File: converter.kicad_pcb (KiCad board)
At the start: 2 copper layers, 26.4 x 49.9 mm, 69 parts, among them CN1 MINI_DIN_8P_JACK, J1 USB_B, J2 USB_microB, SW1 SW_PUSH, U1 ATMEGA32U4, X1 16MHz

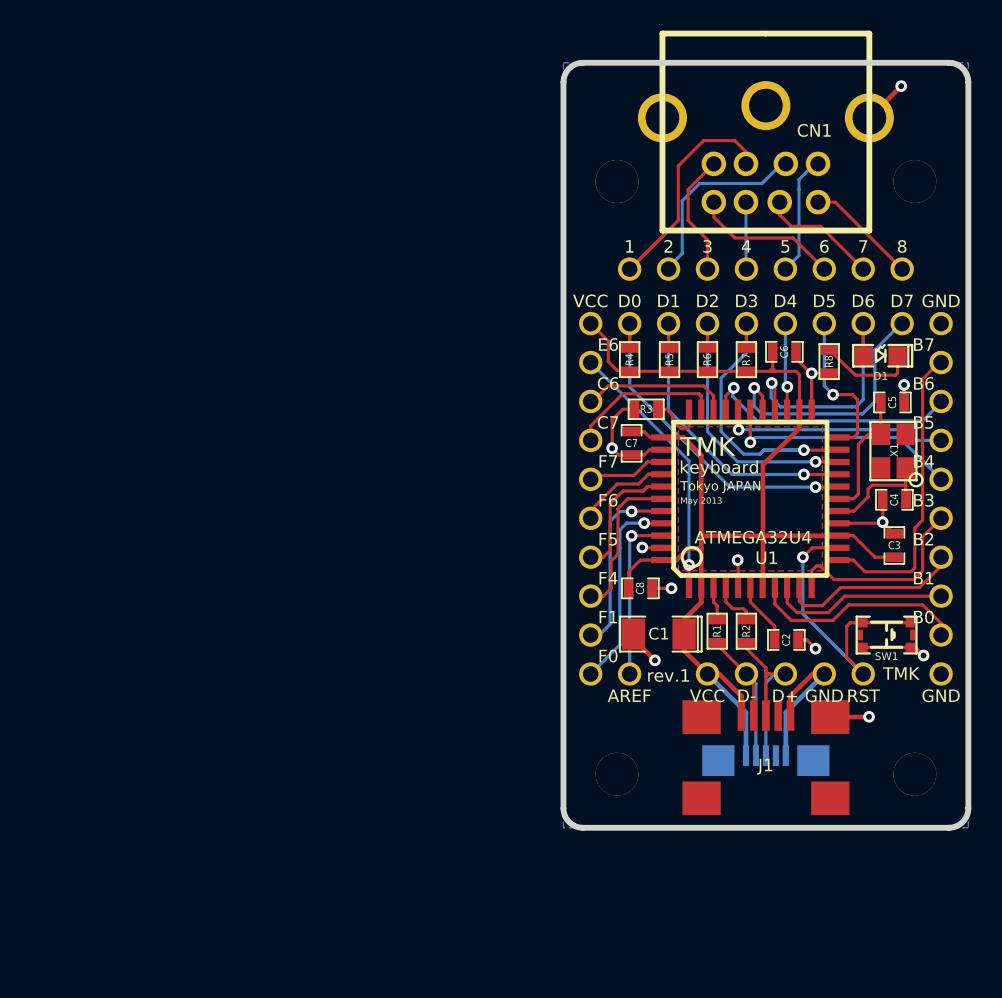
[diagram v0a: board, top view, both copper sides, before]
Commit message: Initial commit of PCB rev.2
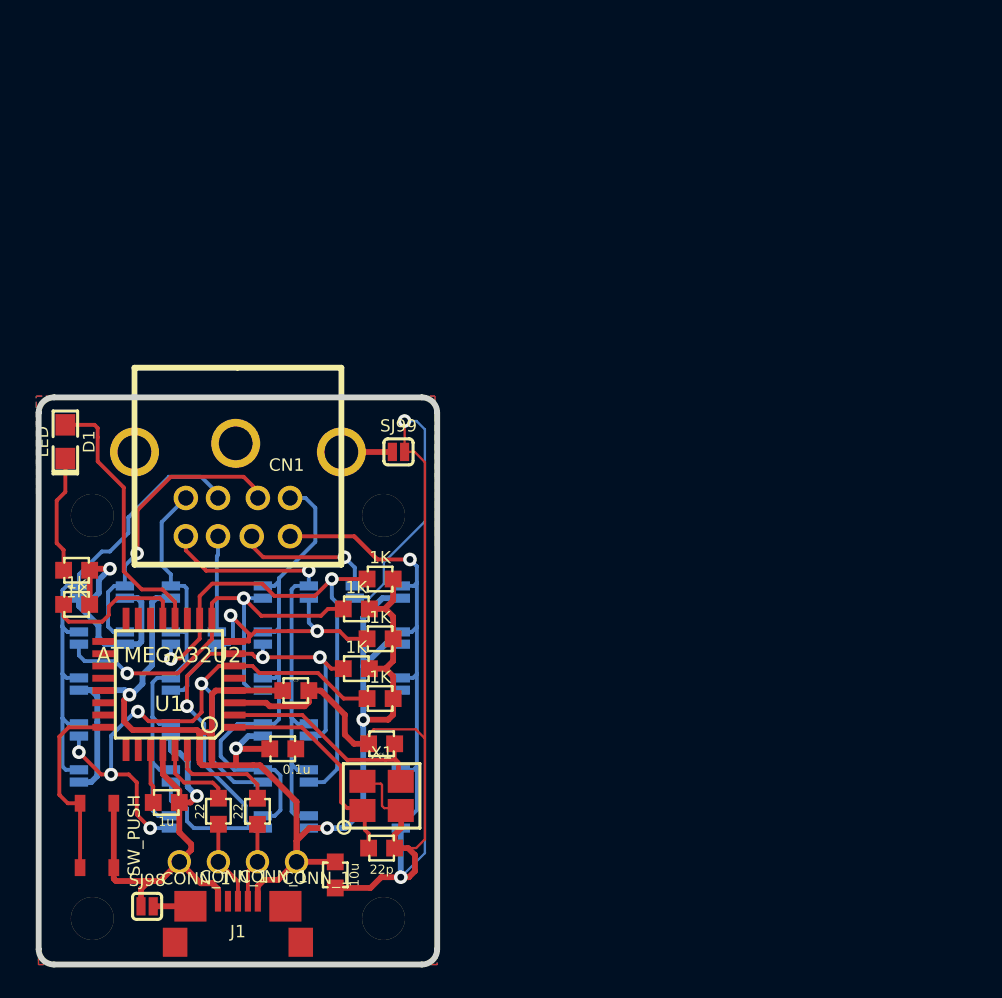
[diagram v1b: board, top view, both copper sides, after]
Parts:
- removed 1, 2, 3, 4, 5, 6, 7, 8, AREF, B0, B1, B2, B3, B4, B5, B6, B7, C7, D+, D-, D0, D2, D3, D4, D5, D6, D7, E6, F0, F1, F4, F5, F6, F7, GND (x3), RST, VCC (x2): CONN_1, PIN_1
- removed the C6 at (136.0, 100.3)
- removed the C6 at (148.7, 97.0)
- removed C7, C8: 0.1u, SM0603_Capa
- removed the D1 at (154.9, 97.3)
- removed the D1 at (141.1, 95.2)
- removed the HOLE_M2.6 at (157.2, 124.6)
- removed the HOLE_M2.6 at (137.7, 85.9)
- removed the HOLE_M2.6 at (157.2, 85.9)
- removed the HOLE_M2.6 at (137.7, 124.6)
- removed J2: USB_microB, USB_microB
- removed R5, R6, R7, R8: 1K, SM0603
- added C6: 22p, 000NewKeyboard_parts:C_1608, F.Cu at (122.4, 122.6)
- added D1: LED, 000NewKeyboard_parts:LED_0805, F.Cu at (101.7, 102.9)
- added HOLE_M2.6: VAL**, HOLE_M2.6, F.Cu at (123.0, 134.0)
- added HOLE_M2.6: VAL**, HOLE_M2.6, F.Cu at (103.4, 107.7)
- added HOLE_M2.6: VAL**, HOLE_M2.6, F.Cu at (122.9, 107.7)
- added HOLE_M2.6: VAL**, HOLE_M2.6, F.Cu at (103.5, 134.0)
- added P1: CONN_1, 000NewKeyboard_parts:PIN_1, F.Cu at (116.8, 130.3)
- added P2: CONN_1, 000NewKeyboard_parts:PIN_1, F.Cu at (114.3, 130.3)
- added P3: CONN_1, 000NewKeyboard_parts:PIN_1, F.Cu at (111.7, 130.3)
- added P4: CONN_1, 000NewKeyboard_parts:PIN_1, F.Cu at (109.2, 130.3)
- added R10: 1K, 000NewKeyboard_parts:R_1608, F.Cu at (122.3, 119.7)
- added R11: 1K, 000NewKeyboard_parts:R_1608, F.Cu at (120.7, 117.7)
- added R12: 1K, 000NewKeyboard_parts:R_1608, F.Cu at (122.3, 115.8)
- added R13: 1K, 000NewKeyboard_parts:R_1608, F.Cu at (120.7, 113.8)
- added R14: 1K, 000NewKeyboard_parts:R_1608, F.Cu at (122.3, 111.8)
- added SJ1: SOLDER_JUMPER, 000NewKeyboard_parts:SOLDER_JUMPER_2, B.Cu at (102.6, 112.7)
- added SJ10: SOLDER_JUMPER, 000NewKeyboard_parts:SOLDER_JUMPER_2, B.Cu at (108.6, 118.7)
- added SJ11: SOLDER_JUMPER, 000NewKeyboard_parts:SOLDER_JUMPER_2, B.Cu at (108.6, 121.7)
- added SJ12: SOLDER_JUMPER, 000NewKeyboard_parts:SOLDER_JUMPER_2, B.Cu at (108.6, 124.7)
- added SJ13: SOLDER_JUMPER, 000NewKeyboard_parts:SOLDER_JUMPER_2, B.Cu at (108.6, 127.7)
- added SJ14: SOLDER_JUMPER, 000NewKeyboard_parts:SOLDER_JUMPER_2, B.Cu at (111.6, 115.7)
- added SJ15: SOLDER_JUMPER, 000NewKeyboard_parts:SOLDER_JUMPER_2, B.Cu at (114.6, 112.7)
- added SJ16: SOLDER_JUMPER, 000NewKeyboard_parts:SOLDER_JUMPER_2, B.Cu at (114.6, 115.7)
- added SJ17: SOLDER_JUMPER, 000NewKeyboard_parts:SOLDER_JUMPER_2, B.Cu at (114.6, 118.7)
- added SJ18: SOLDER_JUMPER, 000NewKeyboard_parts:SOLDER_JUMPER_2, B.Cu at (114.6, 121.7)
- added SJ19: SOLDER_JUMPER, 000NewKeyboard_parts:SOLDER_JUMPER_2, B.Cu at (114.6, 124.7)
- added SJ2: SOLDER_JUMPER, 000NewKeyboard_parts:SOLDER_JUMPER_2, B.Cu at (102.6, 115.7)
- added SJ20: SOLDER_JUMPER, 000NewKeyboard_parts:SOLDER_JUMPER_2, B.Cu at (114.6, 127.7)
- added SJ21: SOLDER_JUMPER, 000NewKeyboard_parts:SOLDER_JUMPER_2, B.Cu at (117.6, 112.7)
- added SJ22: SOLDER_JUMPER, 000NewKeyboard_parts:SOLDER_JUMPER_2, B.Cu at (117.6, 121.7)
- added SJ23: SOLDER_JUMPER, 000NewKeyboard_parts:SOLDER_JUMPER_2, B.Cu at (117.6, 124.7)
- added SJ24: SOLDER_JUMPER, 000NewKeyboard_parts:SOLDER_JUMPER_2, B.Cu at (117.6, 127.7)
- added SJ25: SOLDER_JUMPER, 000NewKeyboard_parts:SOLDER_JUMPER_2, B.Cu at (120.6, 112.7)
- added SJ26: SOLDER_JUMPER, 000NewKeyboard_parts:SOLDER_JUMPER_2, B.Cu at (123.6, 112.7)
- added SJ27: SOLDER_JUMPER, 000NewKeyboard_parts:SOLDER_JUMPER_2, B.Cu at (123.6, 115.7)
- added SJ28: SOLDER_JUMPER, 000NewKeyboard_parts:SOLDER_JUMPER_2, B.Cu at (123.6, 118.7)
- added SJ29: SOLDER_JUMPER, 000NewKeyboard_parts:SOLDER_JUMPER_2, B.Cu at (123.6, 124.7)
- added SJ3: SOLDER_JUMPER, 000NewKeyboard_parts:SOLDER_JUMPER_2, B.Cu at (102.6, 118.7)
- added SJ30: SOLDER_JUMPER, 000NewKeyboard_parts:SOLDER_JUMPER_2, B.Cu at (123.6, 127.7)
- added SJ4: SOLDER_JUMPER, 000NewKeyboard_parts:SOLDER_JUMPER_2, B.Cu at (102.6, 121.7)
- added SJ5: SOLDER_JUMPER, 000NewKeyboard_parts:SOLDER_JUMPER_2, B.Cu at (102.6, 124.7)
- added SJ6: SOLDER_JUMPER, 000NewKeyboard_parts:SOLDER_JUMPER_2, B.Cu at (105.6, 112.7)
- added SJ7: SOLDER_JUMPER, 000NewKeyboard_parts:SOLDER_JUMPER_2, B.Cu at (105.6, 115.7)
- added SJ8: SOLDER_JUMPER, 000NewKeyboard_parts:SOLDER_JUMPER_2, B.Cu at (108.6, 112.7)
- added SJ9: SOLDER_JUMPER, 000NewKeyboard_parts:SOLDER_JUMPER_2, B.Cu at (108.6, 115.7)
- added SJ98: SOLDER_JUMPER, 000NewKeyboard_parts:SOLDER_JUMPER_2, F.Cu at (107.1, 133.2)
- added SJ99: SOLDER_JUMPER, 000NewKeyboard_parts:SOLDER_JUMPER_2, F.Cu at (123.5, 103.6)
- C1: footprint SM1206POL -> 000NewKeyboard_parts:C_1608
- C2, C3, C5: footprint SM0603_Capa -> 000NewKeyboard_parts:C_1608
- C4: value 22p -> 0.1u; footprint SM0603_Capa -> 000NewKeyboard_parts:C_1608
- J1: value USB_B -> USB_mini_micro_B; footprint USB_miniB -> 000NewKeyboard_parts:USB_microB
- R1, R2, R3, R4: footprint SM0603 -> 000NewKeyboard_parts:R_1608
- SW1: footprint SW_ALPS_SKSG -> 000NewKeyboard_parts:SW_ALPS_SKRP
- U1: value ATMEGA32U4 -> ATMEGA32U2; footprint TQFP44 -> 000NewKeyboard_parts:QFP32
- X1: footprint FA-238 -> 000NewKeyboard_parts:FA-238
- moved SW1 53.2 mm to (103.8, 128.6), turned to 90 degrees
- moved C5 44.2 mm to (122.4, 129.4)
- moved C4 43.1 mm to (115.9, 122.9), turned to 0 degrees
- moved C2 41.8 mm to (108.3, 126.4)
- moved CN1 40.8 mm to (113.0, 102.8)
- moved X1 40.3 mm to (122.4, 126.0), turned to 0 degrees
- moved C3 40.2 mm to (116.8, 119.1), turned to 0 degrees
- moved U1 39.8 mm to (108.5, 118.7), turned to 180 degrees
- moved R3 39.3 mm to (102.5, 113.5), turned to 180 degrees
- moved R4 38.6 mm to (102.5, 111.3), turned to 0 degrees
- moved J1 36.5 mm to (113.0, 135.6)
- moved R2 36.4 mm to (111.7, 127.0)
- moved R1 32.2 mm to (114.3, 127.0)
- moved C1 26.3 mm to (119.3, 131.2), turned to 270 degrees
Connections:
- C2 pad 1: N-0000022 -> Net-(C2-Pad1)
- C4 pad 1: N-0000037 -> +5V
- C5 pad 1: N-0000038 -> Net-(C5-Pad1)
- CN1 pad 9: (no net) -> Net-(CN1-Pad9)
- J1 pad 4: (no net) -> Net-(J1-Pad4)
- J1 pad 6: (no net) -> Net-(J1-Pad6)
- R1 pad 1: N-0000025 -> Net-(R1-Pad1)
- R2 pad 1: N-0000024 -> Net-(R2-Pad1)
- R3 pad 2: N-0000013 -> /PD7
- R4 pad 1: +5V -> Net-(D1-Pad2)
- R4 pad 2: /PD0 -> GND
- SW1 pad 1: GND -> /~RESET
- SW1 pad 2: /~RESET -> GND
- U1 pad 1: /PE6 -> Net-(C5-Pad1)
- U1 pad 10: /PB2 -> /PD4
- U1 pad 11: /PB3 -> /PD5
- U1 pad 12: /PB7 -> /PD6
- U1 pad 13: /~RESET -> /PD7
- U1 pad 14: +5V -> /PB0
- U1 pad 15: GND -> /PB1
- U1 pad 16: N-0000037 -> /PB2
- U1 pad 17: N-0000038 -> /PB3
- U1 pad 18: /PD0 -> /PB4
- U1 pad 19: /PD1 -> /PB5
- U1 pad 2: +5V -> Net-(C6-Pad1)
- U1 pad 20: /PD2 -> /PB6
- U1 pad 21: /PD3 -> /PB7
- U1 pad 22: /PD5 -> /PC7
- U1 pad 23: GND -> /PC6
- U1 pad 24: +5V -> /~RESET
- U1 pad 25: /PD4 -> /PC5
- U1 pad 26: /PD6 -> /PC4
- U1 pad 27: /PD7 -> Net-(C2-Pad1)
- U1 pad 28: /PB4 -> GND
- U1 pad 29: /PB5 -> Net-(R2-Pad1)
- U1 pad 3: N-0000025 -> GND
- U1 pad 30: /PB6 -> Net-(R1-Pad1)
- U1 pad 31: /PC6 -> +5V
- U1 pad 32: /PC7 -> +5V
- U1 pad 4: N-0000024 -> +5V
- U1 pad 5: GND -> /PC2
- U1 pad 6: N-0000022 -> /PD0
- U1 pad 7: +5V -> /PD1
- U1 pad 8: /PB0 -> /PD2
- U1 pad 9: /PB1 -> /PD3
- X1 pad 1: N-0000037 -> Net-(C5-Pad1)
- X1 pad 2: N-0000038 -> Net-(C6-Pad1)
- X1 pad 3: (no net) -> GND
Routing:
- net GND: track 51.3 -> 151.1 mm, vias 12 -> 4
- net /PD4: track 5.77 -> 33.0 mm, vias 1 -> 2
- net /DIN8: track 7.30 -> 32.9 mm, vias 0 -> 1
- net /DIN5: track 8.30 -> 33.6 mm
- net +5V: track 83.0 -> 104.4 mm, vias 0 -> 4
- net /PD0: track 22.0 -> 43.2 mm, vias 1 -> 5
- net /DIN3: track 8.09 -> 28.9 mm
- net /DIN6: track 9.59 -> 30.0 mm, vias 0 -> 1
- net /PB7: track 19.6 -> 0.00 mm
- net /PD1: track 20.1 -> 39.1 mm, vias 1 -> 3
- net /PB6: track 17.4 -> 0.00 mm, vias 1 -> 0
- net /PE6: track 17.3 -> 0.00 mm, vias 1 -> 0
- net Net-(C6-Pad1): track 0.00 -> 16.8 mm
- net /PB4: track 15.7 -> 0.00 mm, vias 1 -> 0
- net Net-(C5-Pad1): track 0.00 -> 14.8 mm
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- added copper zone on F.Cu, net GND
- removed copper zone on F.Cu, net +5V
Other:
- board size 26.4 x 49.9 mm -> 26 x 37 mm
- net class 12tho removed
- net class Default: trace_width 0.2032 -> 0.254; via_dia 0.762 -> 0.889
- net class Min6mil added: clearance 0.1524, trace_width 0.1524, via_dia 0.889, via_drill 0.508
- net class Min8mil added: clearance 0.2032, trace_width 0.2032, via_dia 0.889, via_drill 0.508
- net class Power added: clearance 0.254, trace_width 0.381, via_dia 0.889, via_drill 0.508
- rule trace_min: 0.2032 -> 0.1524
- board text added: "1"
- board text added: "2"
- board text added: "3"
- board text added: "4"
- board text added: "5"
- board text added: "6"
- board text added: "7"
- board text added: "8"
- board text added: "ADB"
- board text added: "NEXT"
- board text added: "PC98"
- board text added: "PS/2"
- board text added: "SUN"
- board text added: "X68K"
- board text removed: "May 2013"
- board text removed: "TMK"
- board text removed: "Tokyo JAPAN"
- board text removed: "keyboard"
- board text removed: "rev.1"
